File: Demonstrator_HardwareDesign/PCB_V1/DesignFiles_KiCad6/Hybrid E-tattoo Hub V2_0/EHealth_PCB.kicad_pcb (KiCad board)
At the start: 2 copper layers, 50 x 50 mm, 55 parts, among them J1 Conn_01x06, J2 Conn_01x06, J3 Conn_01x06, J3-MagneticInterconnect1 Conn_01x08, J4 Conn_01x06, J4-OffTheShelf-Digital1 Conn_02x06_Counter_Clockwise, J5-Power1 Conn_01x03, J5-Power2 Conn_01x03, T1 BSC320N20NS3_G, U1 TCA9548APWR, U2 DEBO DCDC DOWN 4

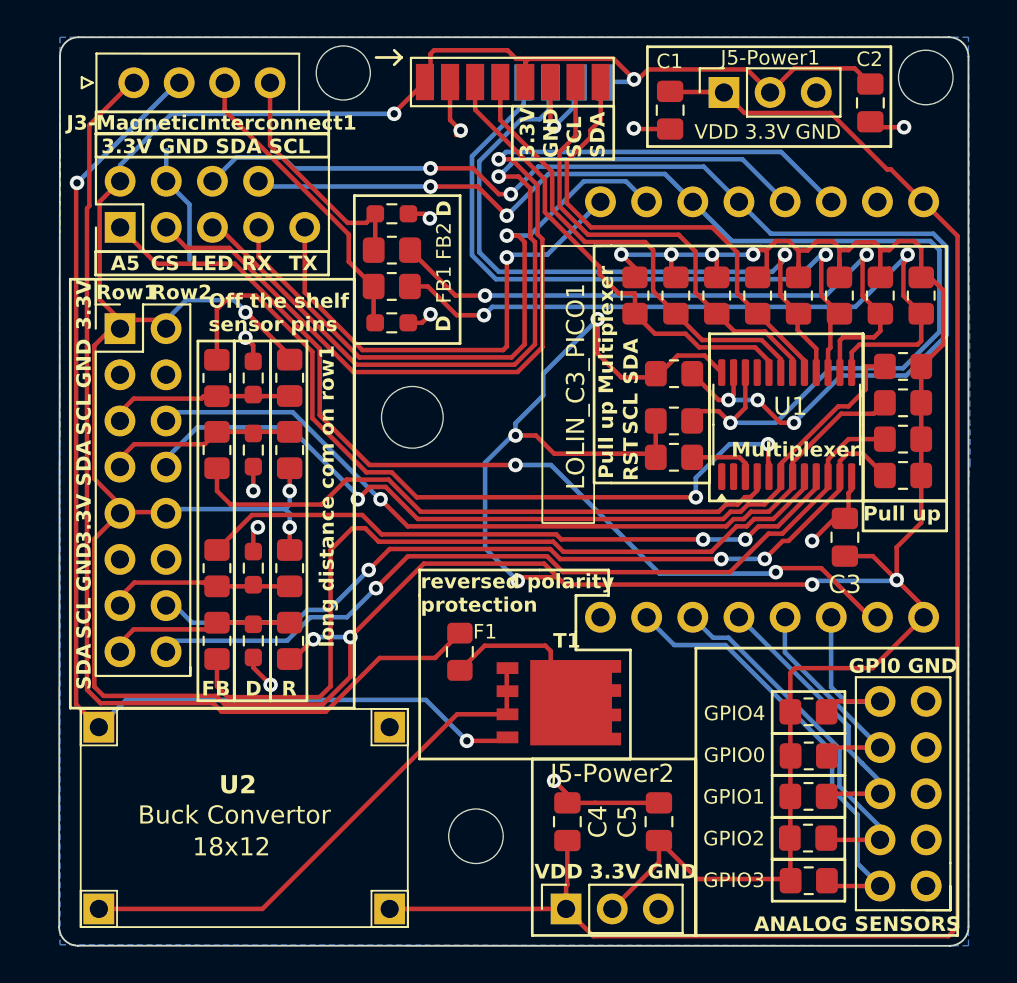
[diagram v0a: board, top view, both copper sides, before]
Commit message: up to date
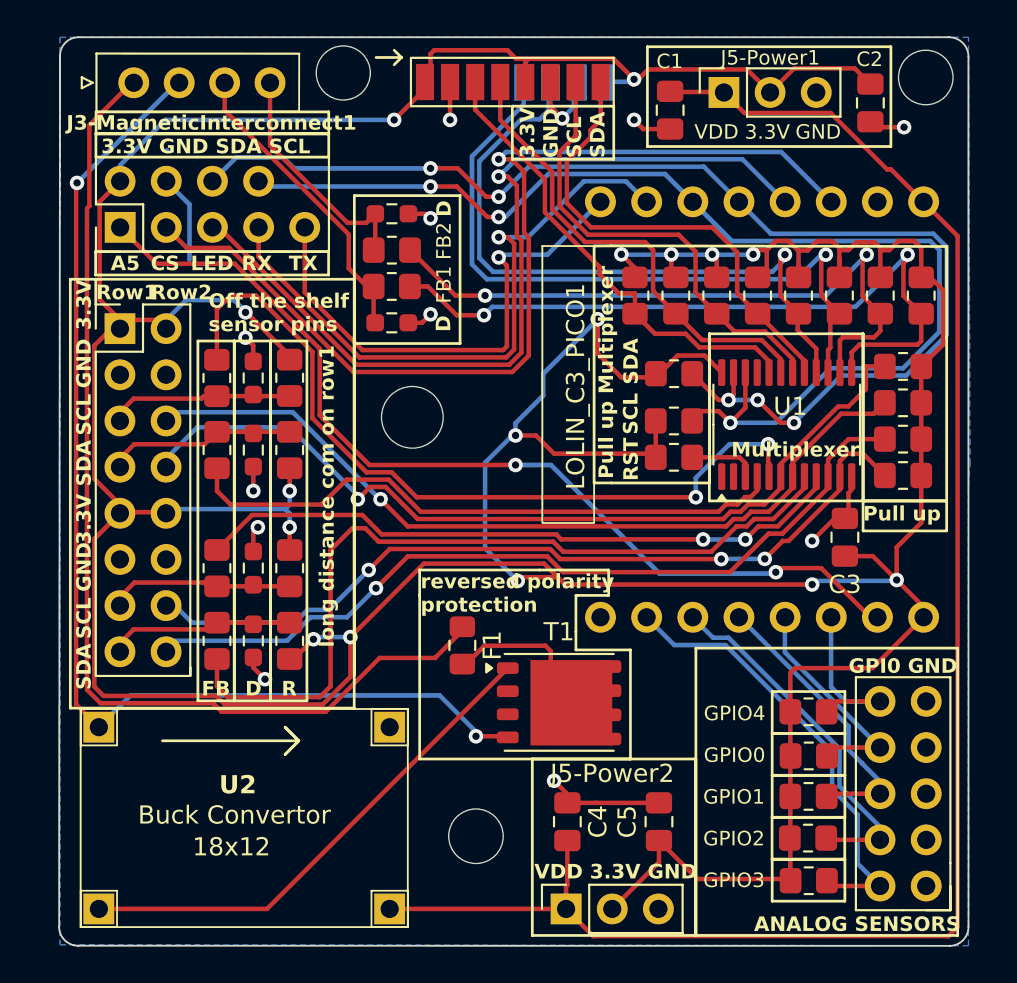
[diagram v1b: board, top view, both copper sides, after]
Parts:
- T1: footprint Library-TRANS:PG-TDSON-8 -> Package_SON:Infineon_PG-TDSON-8_6.15x5.15mm
- moved F1 0.37 mm to (200.8, 89.8)
- turned T1 to 0 degrees
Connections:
- U2 pad 1: Net-(T1-S) -> GND_12V
- U2 pad 2: GND_12V -> Net-(T1-S)
- U2 pad 3: VDD -> GND
- U2 pad 4: GND -> VDD
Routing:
- net GND: track 38.3 -> 34.3 mm
- net Net-(T1-S): track 30.8 -> 28.0 mm
- net /GPIO4_LED: track 49.2 -> 48.0 mm
- net /SPI_CS: track 55.9 -> 55.1 mm
- net /GPIO21_TX: track 27.4 -> 28.0 mm
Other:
- board text removed: "off the shelf sensor pins"
